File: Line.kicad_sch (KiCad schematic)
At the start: 17 parts

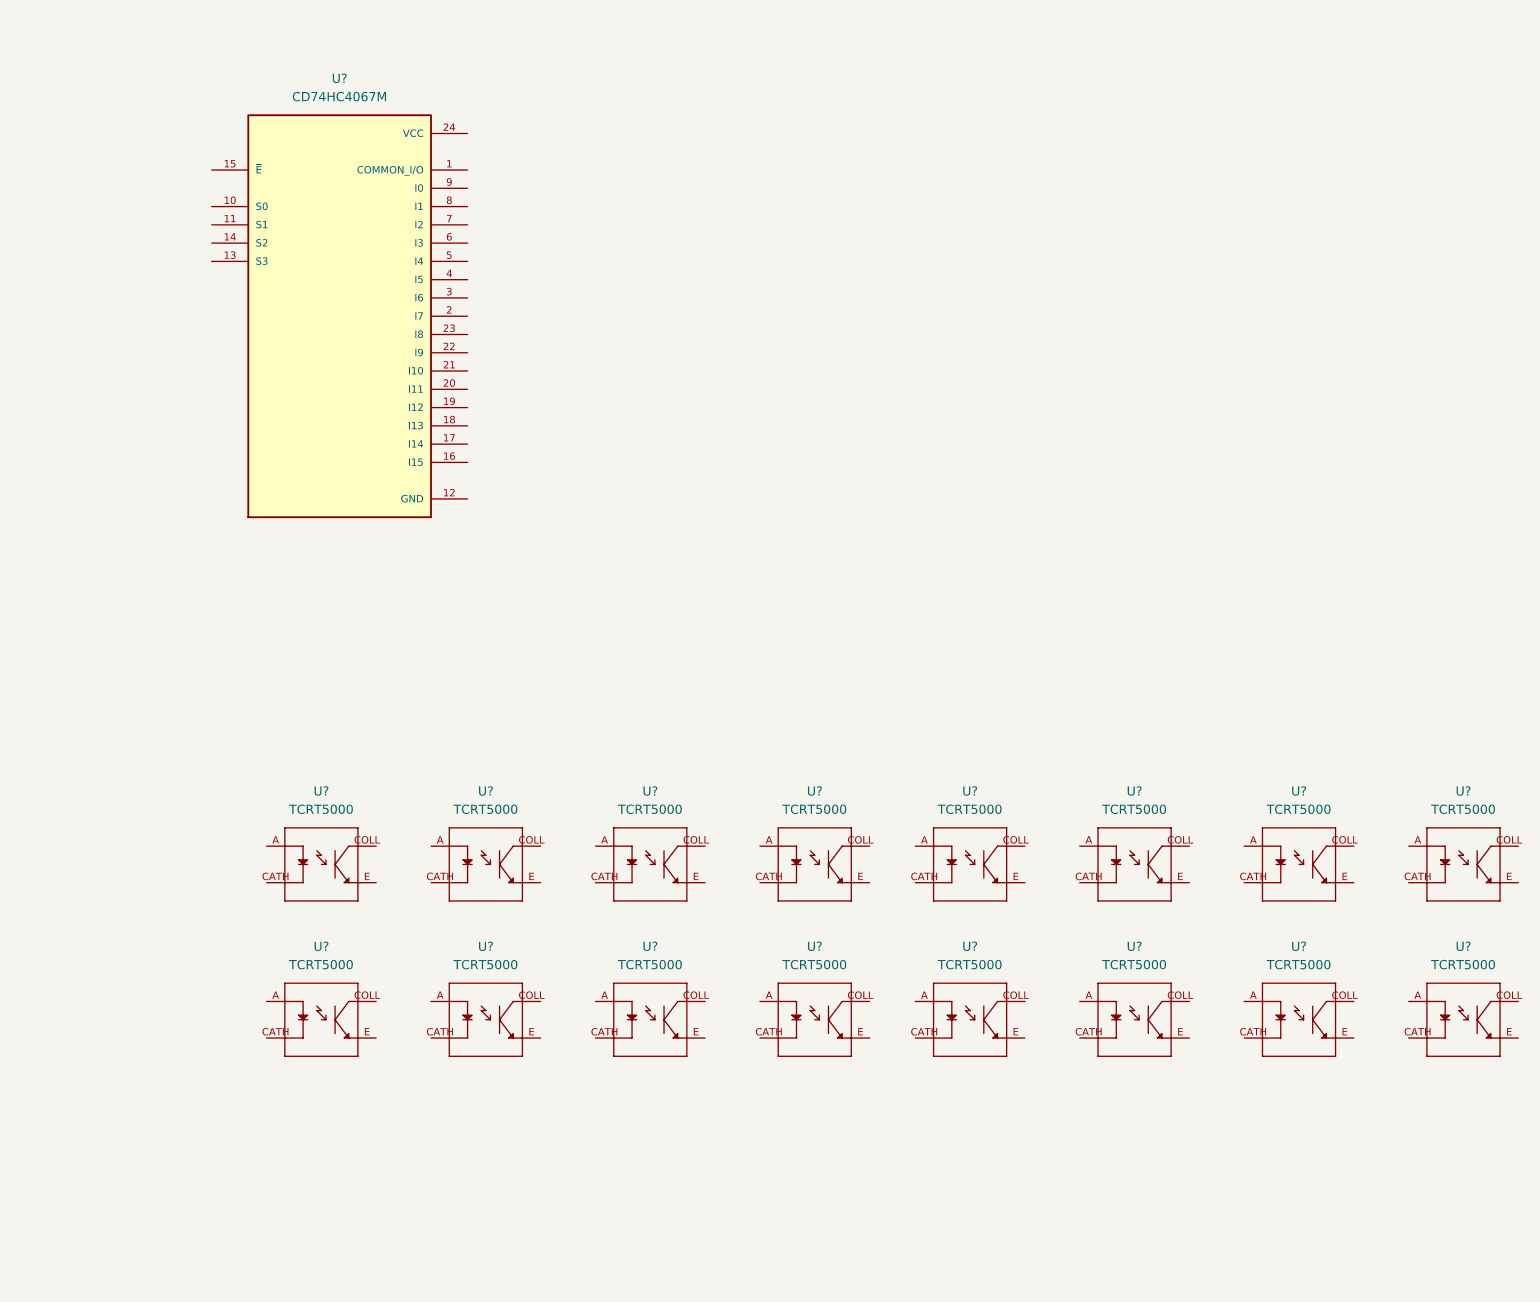
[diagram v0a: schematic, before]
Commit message: schematic
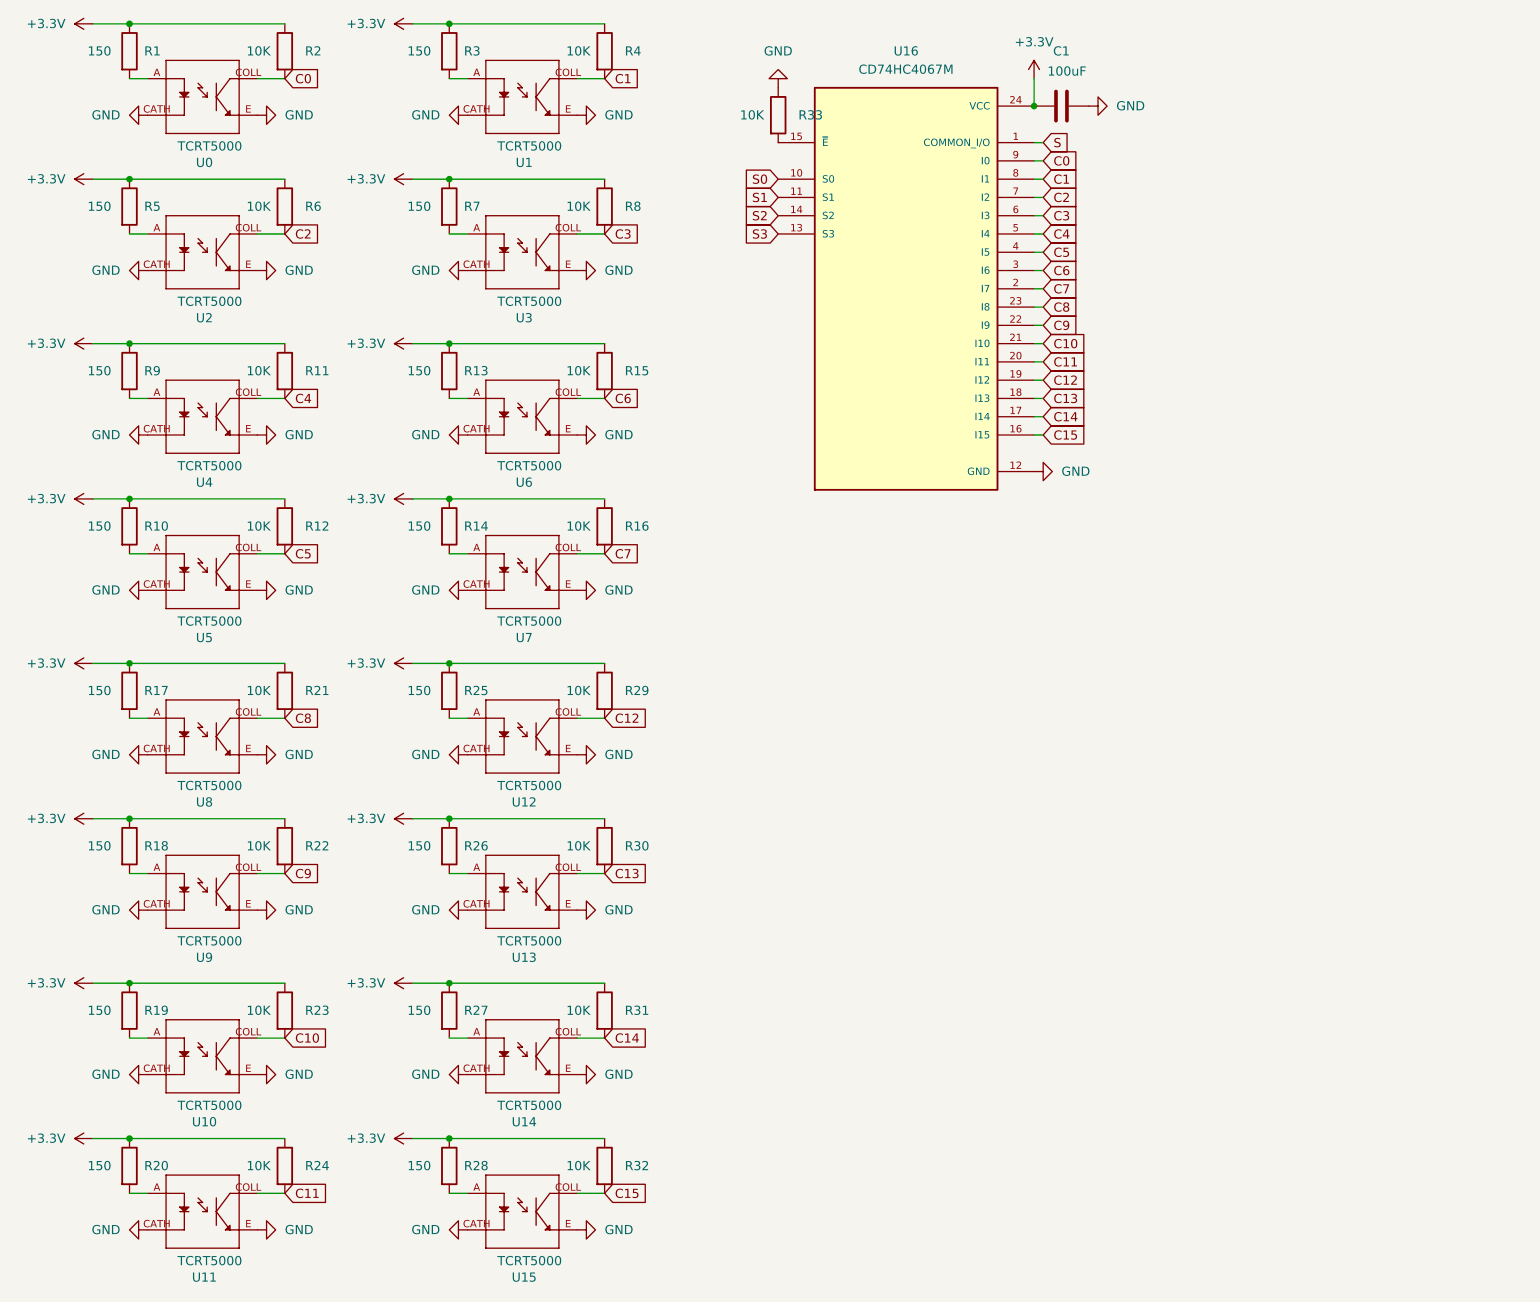
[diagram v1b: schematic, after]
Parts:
- removed U? (x16): TCRT5000, TCRT5000:OPTO_TCRT5000, symbol TCRT5000:TCRT5000
- added C1: 100uF, Capacitor_SMD:C_0603_1608Metric, symbol Device:C
- added R1, R10, R13, R14, R17, R18, R19, R20, R25, R26, R27, R28, R3, R5, R7, R9: 150, Resistor_SMD:R_0805_2012Metric, symbol Device:R
- added R11, R12, R15, R16, R2, R21, R22, R23, R24, R29, R30, R31, R32, R33, R4, R6, R8: 10K, Resistor_SMD:R_0805_2012Metric, symbol Device:R
- added U0, U1, U10, U11, U12, U13, U14, U15, U2, U3, U4, U5, U6, U7, U8, U9: TCRT5000, TCRT5000:OPTO_TCRT5000, symbol TCRT5000:TCRT5000
- gave numbers to parts that had none: 1
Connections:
- net S: now reaches U16.1 (COMMON_I/O)
- net S0: now reaches U16.10 (S0)
- net S1: now reaches U16.11 (S1)
- net GND: now reaches U16.12 (GND)
- net GND: now also C1.2, R33.1, U0.CATH, U0.E, U1.CATH, U1.E, U10.CATH, U10.E, U11.CATH, U11.E, U12.CATH, U12.E, U13.CATH, U13.E, U14.CATH, U14.E, U15.CATH, U15.E, U2.CATH, U2.E, U3.CATH, U3.E, U4.CATH, U4.E, U5.CATH, U5.E, U6.CATH, U6.E, U7.CATH, U7.E, U8.CATH, U8.E, U9.CATH, U9.E
- net S3: now reaches U16.13 (S3)
- net S2: now reaches U16.14 (S2)
- net at U16.15 (~{E}): now also R33.2
- net C15: now reaches U16.16 (I15)
- net C15: now also R32.2, U15.COLL
- net C14: now reaches U16.17 (I14)
- net C14: now also R31.2, U14.COLL
- net C13: now reaches U16.18 (I13)
- net C13: now also R30.2, U13.COLL
- net C12: now reaches U16.19 (I12)
- net C12: now also R29.2, U12.COLL
- net C7: now reaches U16.2 (I7)
- net C7: now also R16.2, U7.COLL
- net C11: now reaches U16.20 (I11)
- net C11: now also R24.2, U11.COLL
- net C10: now reaches U16.21 (I10)
- net C10: now also R23.2, U10.COLL
- net C9: now reaches U16.22 (I9)
- net C9: now also R22.2, U9.COLL
- net C8: now reaches U16.23 (I8)
- net C8: now also R21.2, U8.COLL
- net +3.3V: now reaches U16.24 (VCC)
- net +3.3V: now also C1.1, R1.1, R10.1, R11.1, R12.1, R13.1, R14.1, R15.1, R16.1, R17.1, R18.1, R19.1, R2.1, R20.1, R21.1, R22.1, R23.1, R24.1, R25.1, R26.1, R27.1, R28.1, R29.1, R3.1, R30.1, R31.1, R32.1, R4.1, R5.1, R6.1, R7.1, R8.1, R9.1
- net C6: now reaches U16.3 (I6)
- net C6: now also R15.2, U6.COLL
- net C5: now reaches U16.4 (I5)
- net C5: now also R12.2, U5.COLL
- net C4: now reaches U16.5 (I4)
- net C4: now also R11.2, U4.COLL
- net C3: now reaches U16.6 (I3)
- net C3: now also R8.2, U3.COLL
- net C2: now reaches U16.7 (I2)
- net C2: now also R6.2, U2.COLL
- net C1: now reaches U16.8 (I1)
- net C1: now also R4.2, U1.COLL
- net C0: now reaches U16.9 (I0)
- net C0: now also R2.2, U0.COLL
- new net: R19.2, U10.A
- new net: R14.2, U7.A
- new net: R26.2, U13.A
- new net: R7.2, U3.A
- new net: R17.2, U8.A
- new net: R25.2, U12.A
- new net: R18.2, U9.A
- new net: R27.2, U14.A
- new net: R3.2, U1.A
- new net: R5.2, U2.A
- new net: R28.2, U15.A
- new net: R1.2, U0.A
- new net: R9.2, U4.A
- new net: R13.2, U6.A
- new net: R10.2, U5.A
- new net: R20.2, U11.A
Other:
- moved on the sheet: U16
